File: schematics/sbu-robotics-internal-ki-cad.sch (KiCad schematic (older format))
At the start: 6 parts, among them M1 Motor_DC, M2 Motor_DC

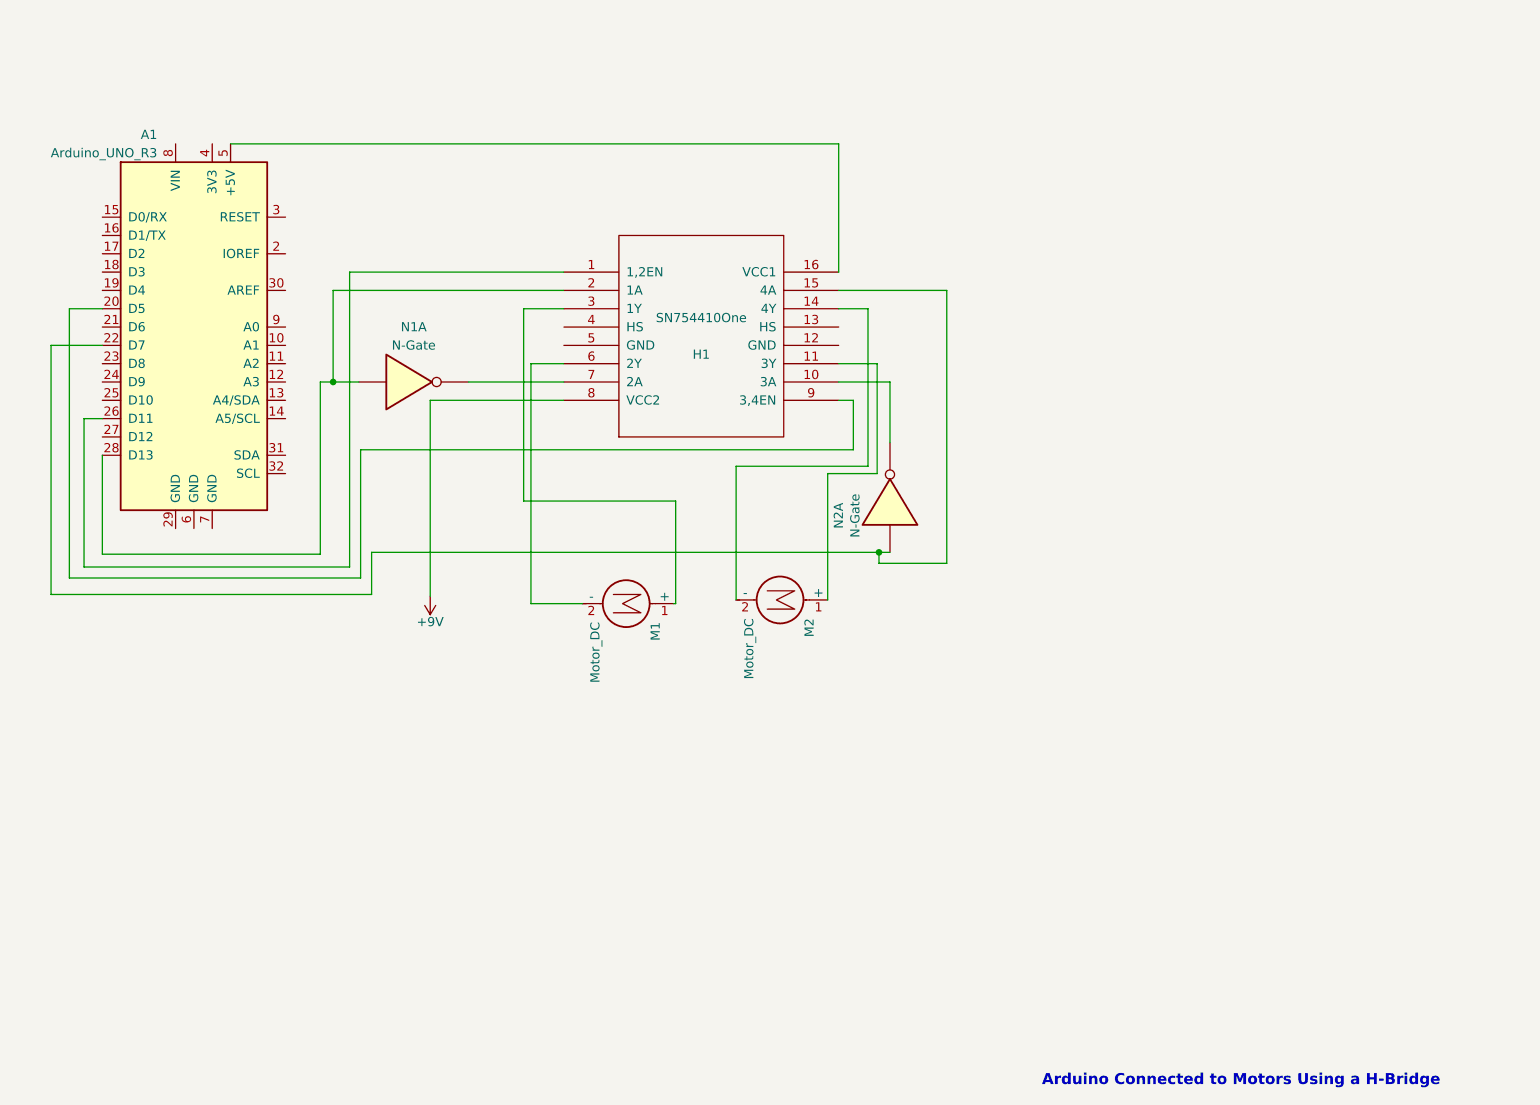
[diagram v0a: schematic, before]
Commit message: Add files via upload
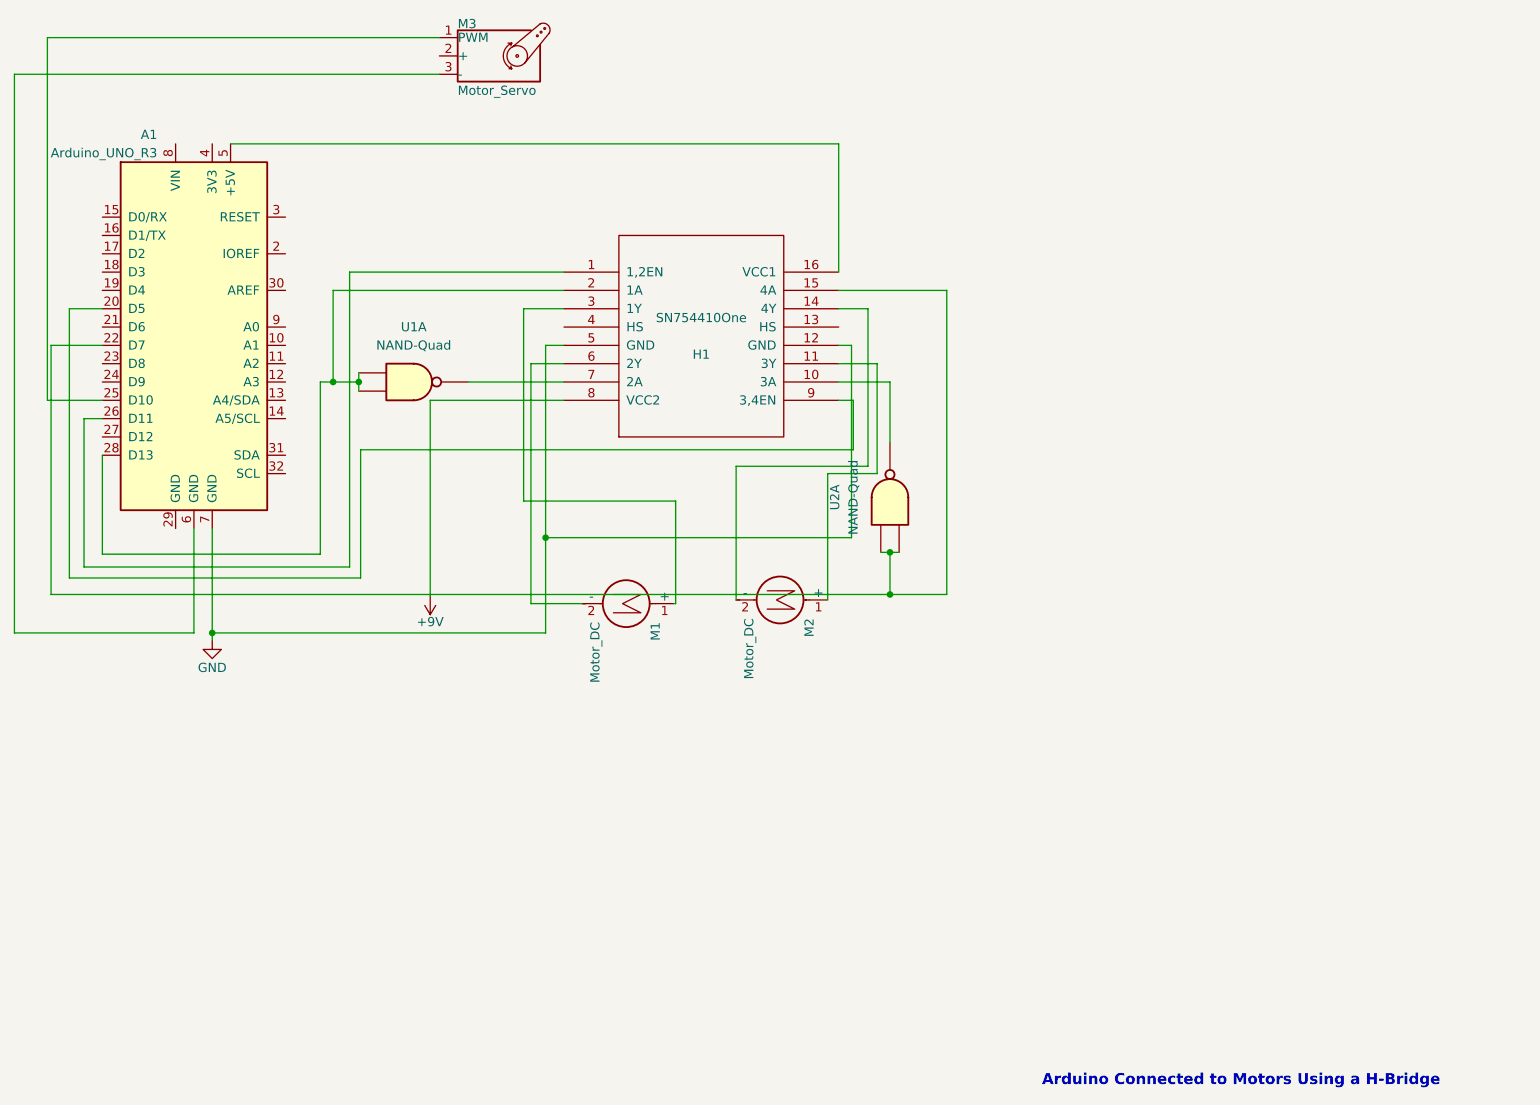
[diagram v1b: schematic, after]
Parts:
- removed N1, N2: N-Gate, footprint, symbol NOT-Hex
- added M3: Motor_Servo, symbol Motor_Servo
- added U1, U2: NAND-Quad, footprint, symbol NAND-Quad
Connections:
- net at H1.10 (3A): now also U2.~ (QA)
- net GND: now reaches H1.12 (GND)
- net GND: now also A1.7 (GND), H1.5 (GND)
- net at A1.22 (D7), H1.15 (4A): now also U2.~ (QA)
- net at A1.28 (D13), H1.2 (1A): now also U1.~ (QA)
- net at H1.7 (2A): now also U1.~ (QA)
- net at A1.25 (D10): now also M3.1 (PWM)
- net at A1.6 (GND): now also M3.3 (-)
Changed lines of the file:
@@
-	1    0    0    -1
-$EndComp
-$Comp
-L NOT-Hex N2
-U 1 1 59E0235E
-P 6560 4280
-F 0 "N2" H 6460 4560 50  0000 C CNN
-F 1 "N-Gate" H 6460 4470 50  0000 C CNN
-F 2 "footprint" H 6560 3280 50  0001 C CNN
-F 3 "datasheet" H 6560 3180 50  0001 C CNN
-F 4 "bom" H 6560 3080 50  0001 C CNN "BOM"
-	1    6560 4280
-	0    -1   -1   0
-$EndComp
-$Comp
-L NOT-Hex N1
-U 1 1 59E02C01
-P 3960 3650
-F 0 "N1" H 3960 3950 50  0000 C CNN
-F 1 "N-Gate" H 3960 3850 50  0000 C CNN
-F 2 "footprint" H 3960 2650 50  0001 C CNN
-F 3 "datasheet" H 3960 2550 50  0001 C CNN
-F 4 "bom" H 3960 2450 50  0001 C CNN "BOM"
-	1    3960 3650
 	1    0    0    -1
 $EndComp
@@
 	1980 3450 1980 4810
 Wire Wire Line
-	1980 4810 3730 4810
-Wire Wire Line
-	3730 4810 3730 4580
-Wire Wire Line
-	3730 4580 6560 4580
-Wire Wire Line
-	6500 4580 6500 4640
-Wire Wire Line
-	6500 4640 6870 4640
-Wire Wire Line
-	6870 4640 6870 3150
+	1980 4810 6870 4810
 Wire Wire Line
 	6870 3150 6280 3150
-Connection ~ 6500 4580
 Wire Wire Line
 	6560 3980 6560 3650
@@
 Arduino Connected to Motors Using a H-Bridge\n
 $Comp
-L +9V #PWR?
+L +9V #PWR2
 U 1 1 59E05DE5
 P 4050 4820
-F 0 "#PWR?" H 4050 4670 50  0001 C CNN
+F 0 "#PWR2" H 4050 4670 50  0001 C CNN
 F 1 "+9V" H 4050 4960 50  0000 C CNN
 F 2 "" H 4050 4820 50  0001 C CNN
@@
 Wire Wire Line
 	4050 3750 4050 4820
+$Comp
+L GND #PWR1
+U 1 1 59E10209
+P 2860 5060
+F 0 "#PWR1" H 2860 4810 50  0001 C CNN
+F 1 "GND" H 2860 4910 50  0000 C CNN
+F 2 "" H 2860 5060 50  0001 C CNN
+F 3 "" H 2860 5060 50  0001 C CNN
+	1    2860 5060
+	1    0    0    -1
+$EndComp
+Wire Wire Line
+	2860 5060 2860 4450
+$Comp
+L NAND-Quad U1
+U 1 1 59E26706
+P 3960 3650
+F 0 "U1" H 3960 3950 50  0000 C CNN
+F 1 "NAND-Quad" H 3960 3850 50  0000 C CNN
+F 2 "footprint" H 3960 2750 50  0001 C CNN
+F 3 "datasheet" H 3960 2650 50  0001 C CNN
+F 4 "bom" H 3960 2550 50  0001 C CNN "BOM"
+	1    3960 3650
+	1    0    0    -1
+$EndComp
+Wire Wire Line
+	3660 3600 3660 3700
+$Comp
+L NAND-Quad U2
+U 1 1 59E26C1C
+P 6560 4280
+F 0 "U2" H 6560 4580 50  0000 C CNN
+F 1 "NAND-Quad" H 6560 4480 50  0000 C CNN
+F 2 "footprint" H 6560 3380 50  0001 C CNN
+F 3 "datasheet" H 6560 3280 50  0001 C CNN
+F 4 "bom" H 6560 3180 50  0001 C CNN "BOM"
+	1    6560 4280
+	0    -1   -1   0
+$EndComp
+Wire Wire Line
+	6560 4810 6560 4580
+Wire Wire Line
+	6510 4580 6610 4580
+Connection ~ 6560 4580
+Wire Wire Line
+	6870 4810 6870 3150
+Connection ~ 6560 4810
+Connection ~ 3660 3650
+Wire Wire Line
+	2860 5020 4680 5020
+Wire Wire Line
+	4680 5020 4680 3450
+Wire Wire Line
+	4680 3450 4780 3450
+Connection ~ 2860 5020
+Wire Wire Line
+	4680 4500 6350 4500
+Wire Wire Line
+	6350 4500 6350 3450
+Wire Wire Line
+	6350 3450 6280 3450
+Connection ~ 4680 4500
+$Comp
+L Motor_Servo M3
+U 1 1 59E29295
+P 4400 1870
+F 0 "M3" H 4200 2045 50  0000 L CNN
+F 1 "Motor_Servo" H 4200 1710 50  0000 L TNN
+F 2 "" H 4400 1680 50  0001 C CNN
+F 3 "" H 4400 1680 50  0001 C CNN
+	1    4400 1870
+	1    0    0    -1
+$EndComp
+Wire Wire Line
+	4100 1770 1960 1770
+Wire Wire Line
+	1960 1770 1960 3750
+Wire Wire Line
+	1960 3750 2260 3750
+Wire Wire Line
+	1780 1970 4100 1970
+Wire Wire Line
+	1780 1970 1780 5020
+Wire Wire Line
+	1780 5020 2760 5020
+Wire Wire Line
+	2760 5020 2760 4450
 $EndSCHEMATC
